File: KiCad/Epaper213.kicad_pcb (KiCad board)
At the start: 2 copper layers, 43.2 x 43.2 mm, 34 parts, among them J1 USB-C, J2 DC, J3 Conn_01x02, M1 EPaper, U1 LMR16006+FB, U2 FT231XQ, U3 ESP32-PICO-MINI-02, U4 QR

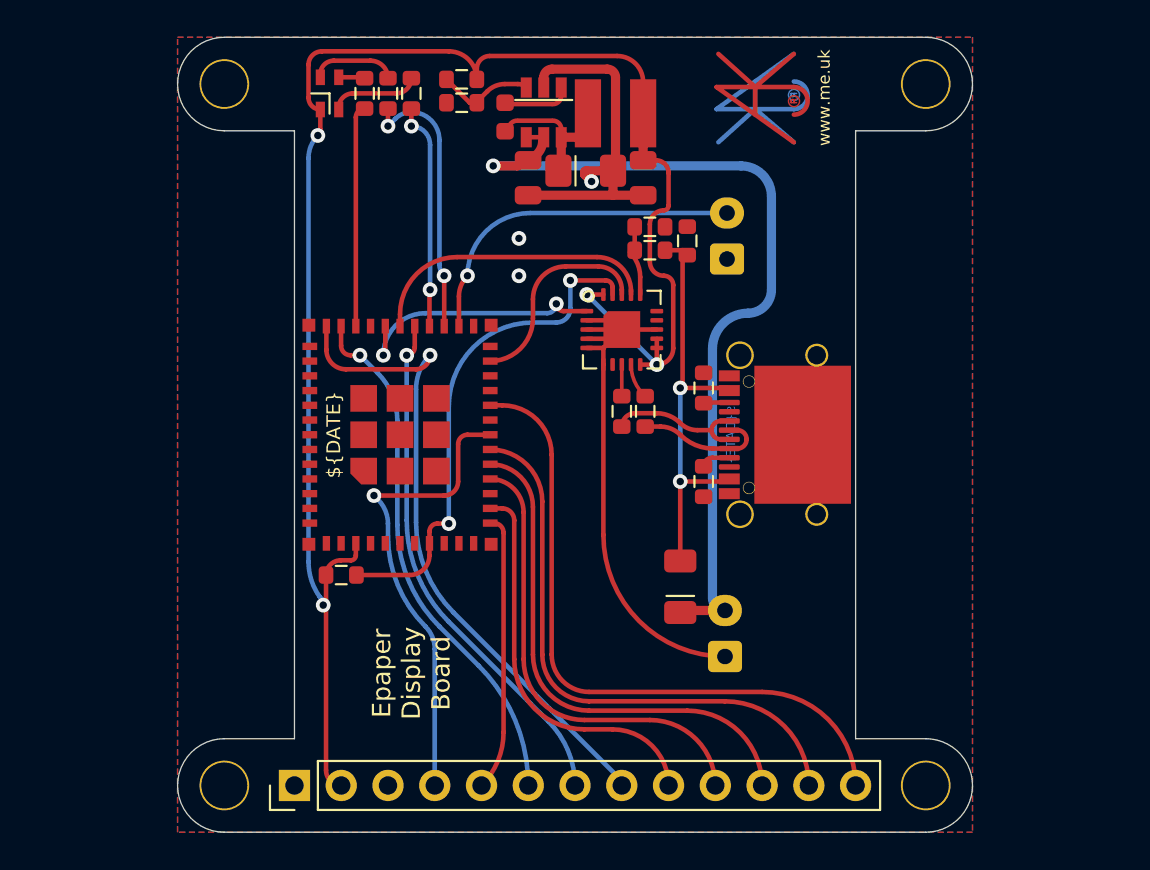
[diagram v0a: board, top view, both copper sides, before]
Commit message: Both epaper boards
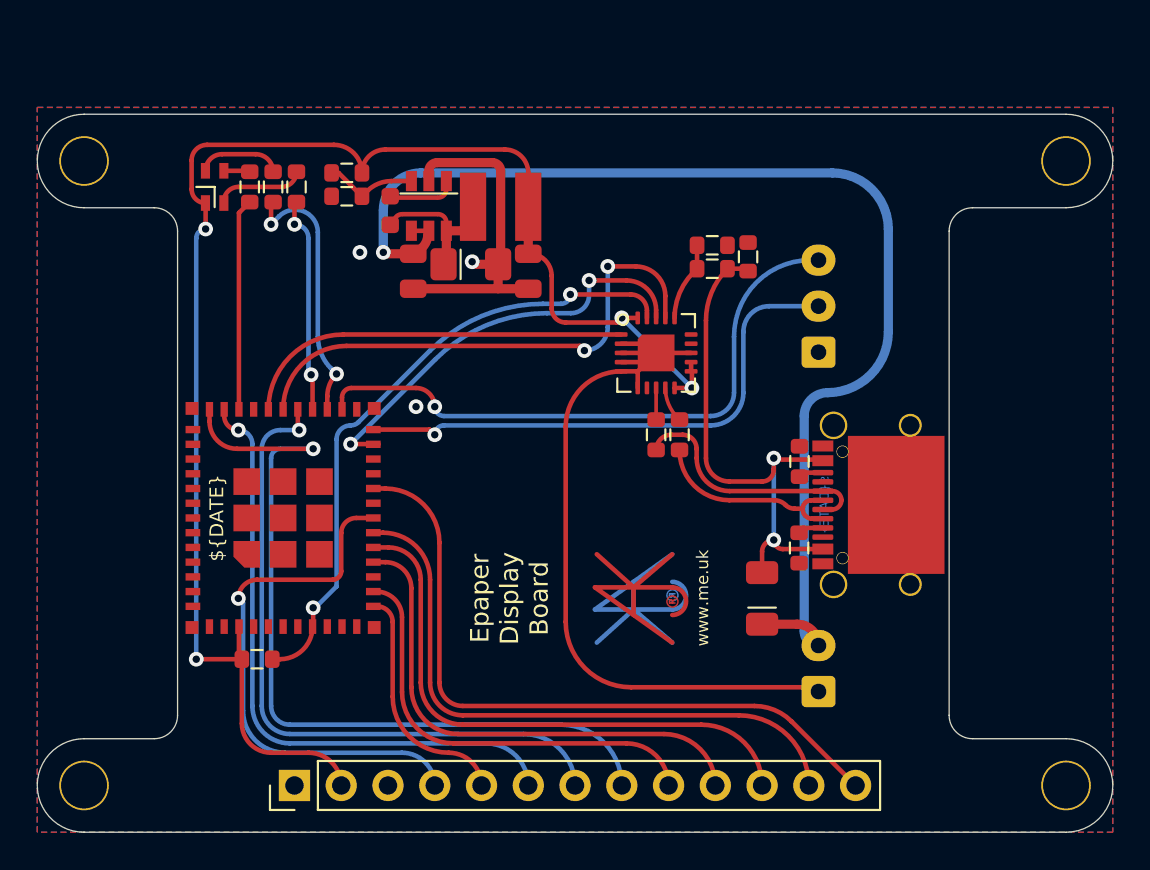
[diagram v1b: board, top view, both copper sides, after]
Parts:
- J3: footprint RevK:Molex_MiniSPOX_H2RA -> RevK:Molex_MiniSPOX_H3RA
- moved Logo2 28.0 mm to (154.3, 92.0)
- moved Logo1 28.0 mm to (154.3, 90.8)
- moved H2 8.69 mm to (124.5, 67.7)
- moved H1 8.69 mm to (177.8, 67.7)
- moved R10 8.05 mm to (134.7, 69.1)
- moved R12 8.05 mm to (136.0, 69.1)
- moved R2 8.05 mm to (138.7, 69.6)
- moved U1 8.05 mm to (143.2, 70.1)
- moved R1 8.05 mm to (138.7, 68.3)
- moved D3 8.05 mm to (131.6, 69.1)
- moved R11 8.05 mm to (133.5, 69.1)
- moved U3 7.79 mm to (135.3, 87.1)
- moved H3 7.62 mm to (124.5, 101.6)
- moved H4 7.62 mm to (177.8, 101.6)
- moved R4 6.56 mm to (163.3, 84.0)
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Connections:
- J3 pad 2: BUTTON -> BUTTON1
- U3 pad 24: unconnected-(U3-Pad24) -> BUTTON1
- U3 pad 26: BUTTON -> BUTTON2
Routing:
- net BUTTON2: track 0.00 -> 33.5 mm, vias 0 -> 1
- net BUTTON1: track 0.00 -> 29.6 mm, vias 0 -> 1
- net BUTTON: track 18.8 -> 0.00 mm, vias 1 -> 0
- net DC: track 45.8 -> 64.2 mm
- net I: track 16.0 -> 28.7 mm, vias 0 -> 2
- net BOOT: track 11.3 -> 23.3 mm, vias 0 -> 2
- net GND: track 32.1 -> 43.0 mm
- net D/C: track 35.7 -> 44.4 mm
- net CS: track 28.4 -> 37.0 mm
- net +3V3: track 90.0 -> 82.1 mm
- net EN: track 27.3 -> 34.6 mm
- net O: track 14.4 -> 21.3 mm, vias 2 -> 0
- net Net-(J1-PadA6): track 7.95 -> 13.9 mm
- net VBUS: track 23.4 -> 29.3 mm
- net MOSI: track 28.5 -> 34.2 mm
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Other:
- board size 43.2 x 43.2 mm -> 58.4 x 39 mm
- board text added: "4"
- board text added: "⏚"
